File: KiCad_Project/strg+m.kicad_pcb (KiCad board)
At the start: 2 copper layers, 37.9 x 91.4 mm, 40 parts, among them J1 Conn_01x04_Female, J10 Conn_01x03_Male, J11 Conn_01x02_Male, J2 Conn_01x03_Female, J3 Conn_01x03_Female, J4 Conn_01x02_Female, J5 AudioJack2, J6 AudioJack2, J7 Conn_02x05_Odd_Even, J8 Conn_01x04_Male, J9 Conn_01x03_Male, U1 LM324

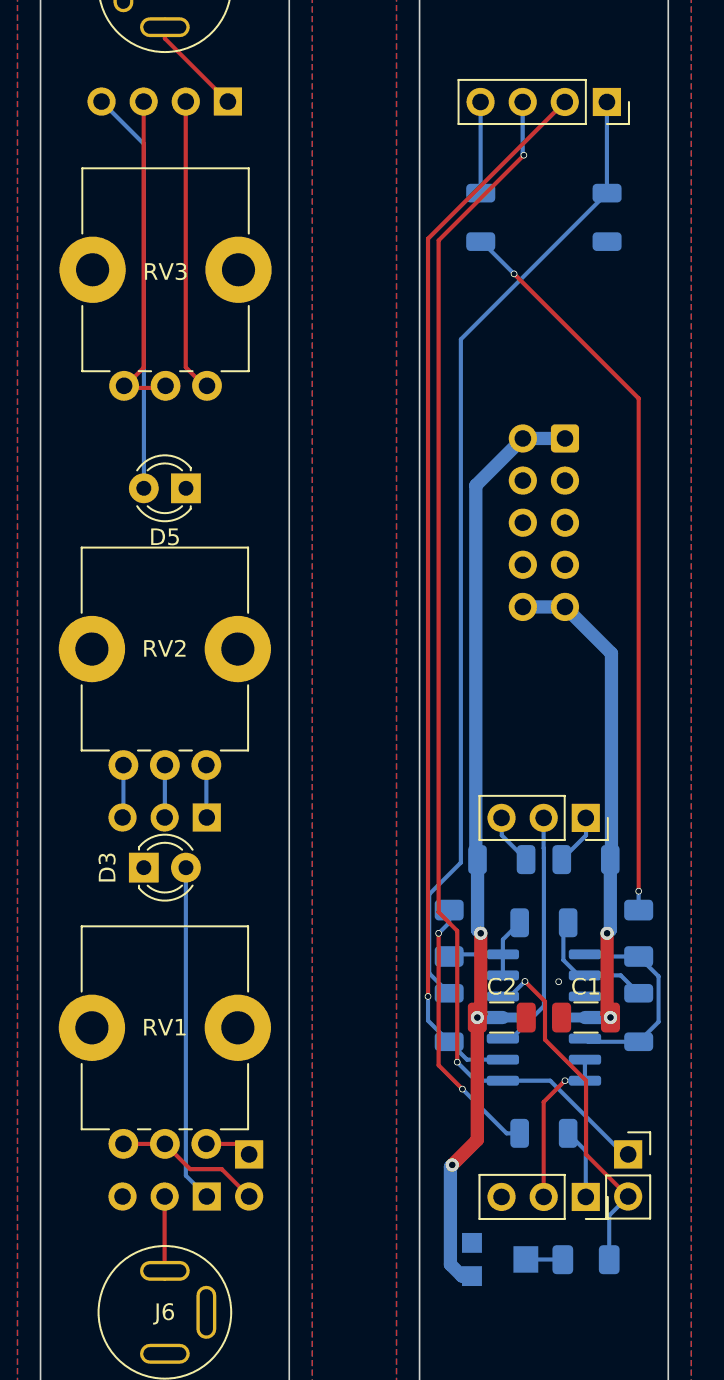
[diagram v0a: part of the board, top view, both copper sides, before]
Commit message: update pcb layout
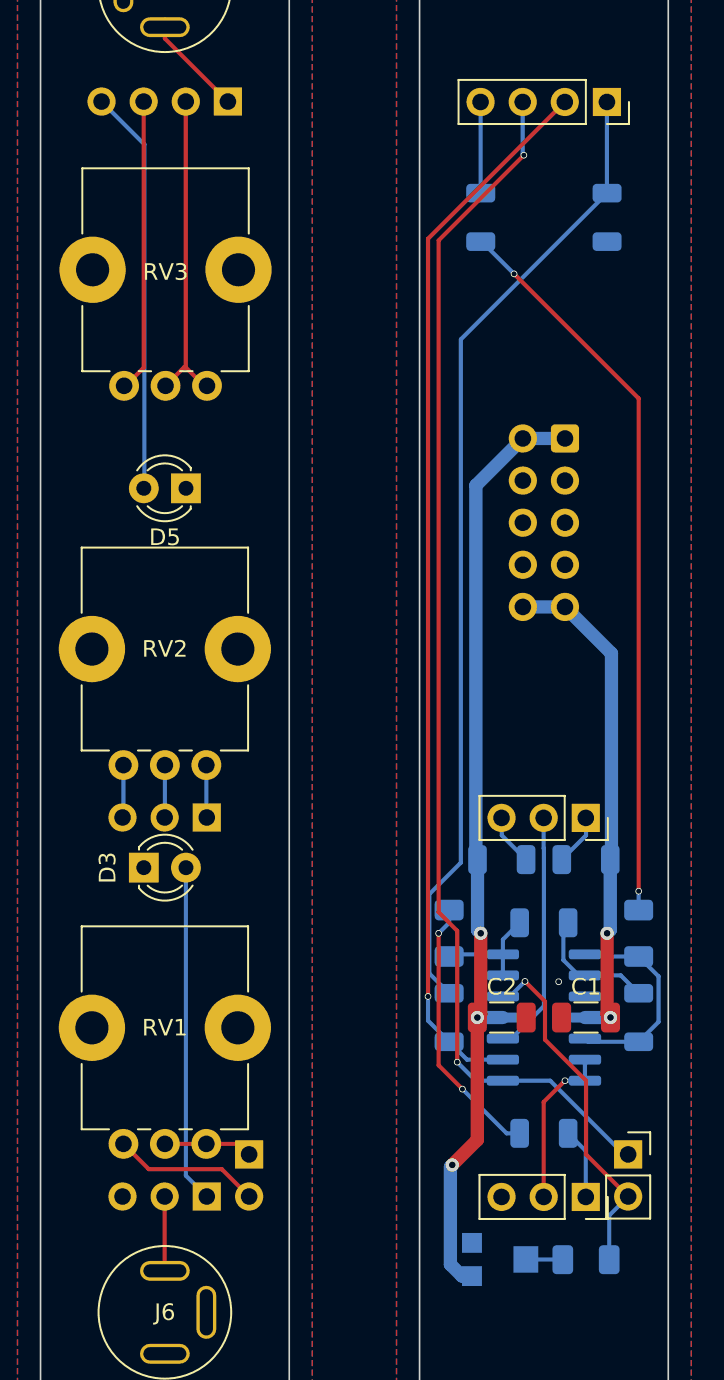
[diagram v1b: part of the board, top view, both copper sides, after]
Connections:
- net /ctrl+m interface/0V renamed /strg+m interface/0V
- net /ctrl+m interface/cv_in renamed /strg+m interface/cv_in
- net /ctrl+m interface/cv_out renamed /strg+m interface/cv_out
- net /ctrl+m interface/neg_halfwave renamed /strg+m interface/neg_halfwave
- net /ctrl+m interface/offset_left renamed /strg+m interface/offset_left
- net /ctrl+m interface/offset_middle renamed /strg+m interface/offset_middle
- net /ctrl+m interface/offset_right renamed /strg+m interface/offset_right
- net /ctrl+m interface/pos_halfwave renamed /strg+m interface/pos_halfwave
- net /ctrl+m main pcb/clip_left renamed /strg+m main pcb/clip_left
- net /ctrl+m main pcb/clip_right renamed /strg+m main pcb/clip_right
- net /ctrl+m main pcb/cv_in renamed /strg+m main pcb/cv_in
- net /ctrl+m main pcb/cv_out renamed /strg+m main pcb/cv_out
- net /ctrl+m main pcb/neg_halfwave renamed /strg+m main pcb/neg_halfwave
- net /ctrl+m main pcb/offset_left renamed /strg+m main pcb/offset_left
- net /ctrl+m main pcb/offset_middle renamed /strg+m main pcb/offset_middle
- net /ctrl+m main pcb/offset_right renamed /strg+m main pcb/offset_right
- net /ctrl+m main pcb/pos_halfwave renamed /strg+m main pcb/pos_halfwave
- net /ctrl+m main pcb/range_left renamed /strg+m main pcb/range_left
- J1 pad 2: /ctrl+m interface/range_left -> /strg+m interface/range_left
- J1 pad 3: /ctrl+m interface/range_right -> /strg+m interface/range_right
- J4 pad 1: /ctrl+m interface/clip_left -> /strg+m interface/clip_left
- J4 pad 2: /ctrl+m interface/clip_right -> /strg+m interface/clip_right
- RV1 pad 1: /ctrl+m interface/clip_left -> /strg+m interface/clip_left
- RV1 pad 2: /ctrl+m interface/clip_right -> /strg+m interface/clip_left
- RV1 pad 3: /ctrl+m interface/clip_right -> /strg+m interface/clip_right
- RV3 pad 1: /ctrl+m interface/range_left -> /strg+m interface/range_left
- RV3 pad 2: /ctrl+m interface/range_right -> /strg+m interface/range_left
- RV3 pad 3: /ctrl+m interface/range_right -> /strg+m interface/range_right
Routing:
- net /ctrl+m interface/range_right: track 20.3 -> 0.00 mm
- net /strg+m interface/range_left: track 0.00 -> 19.5 mm
- net /ctrl+m interface/range_left: track 17.8 -> 0.00 mm
- net /strg+m interface/range_right: track 0.00 -> 17.8 mm
- net /strg+m interface/clip_right: track 0.00 -> 8.90 mm
- net /ctrl+m interface/clip_right: track 8.90 -> 0.00 mm
- net /strg+m interface/clip_left: track 0.00 -> 5.34 mm
- net /ctrl+m interface/clip_left: track 2.84 -> 0.00 mm
- net /strg+m interface/pos_halfwave: track 23.9 -> 24.4 mm
